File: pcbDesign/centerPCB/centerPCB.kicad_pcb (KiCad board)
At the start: 2 copper layers, 157 x 58.8 mm, 11 parts, among them J1 Conn_01x07_Pin, J2 Conn_01x12_Pin

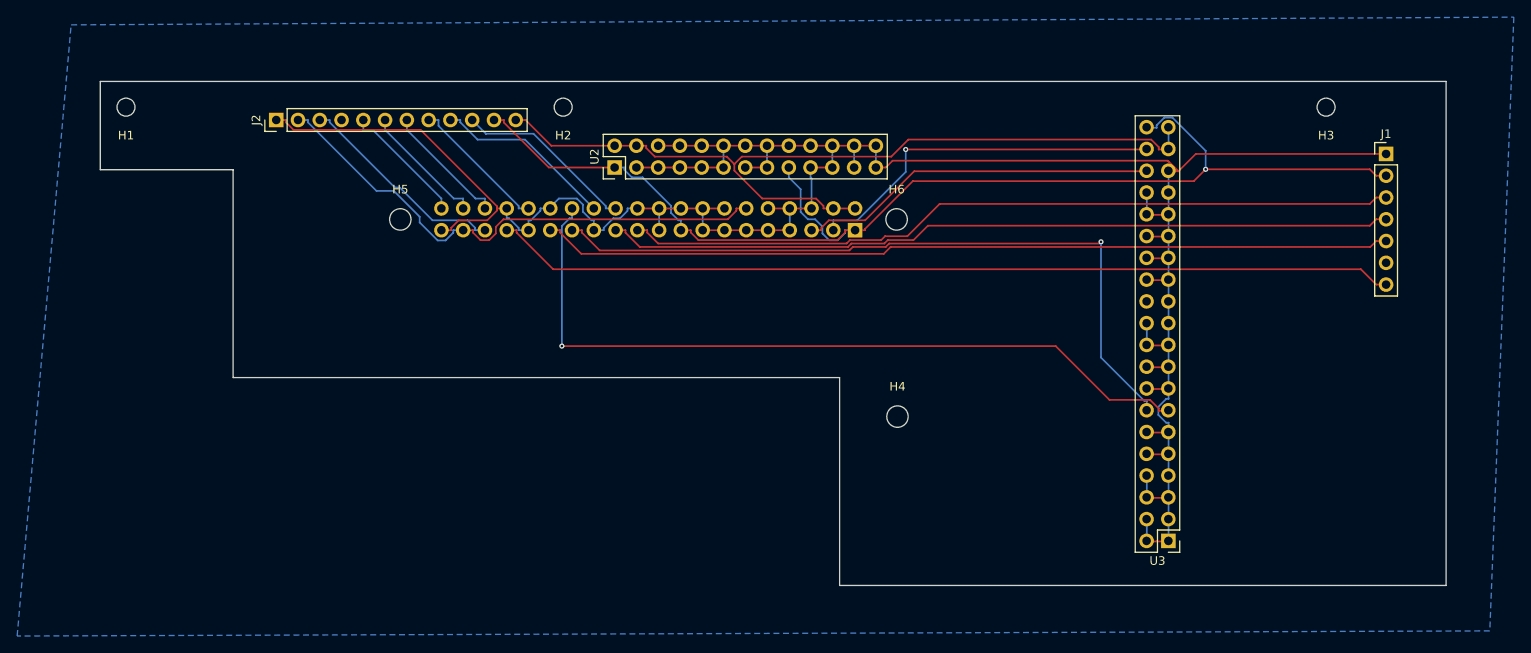
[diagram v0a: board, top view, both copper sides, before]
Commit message: rerouted
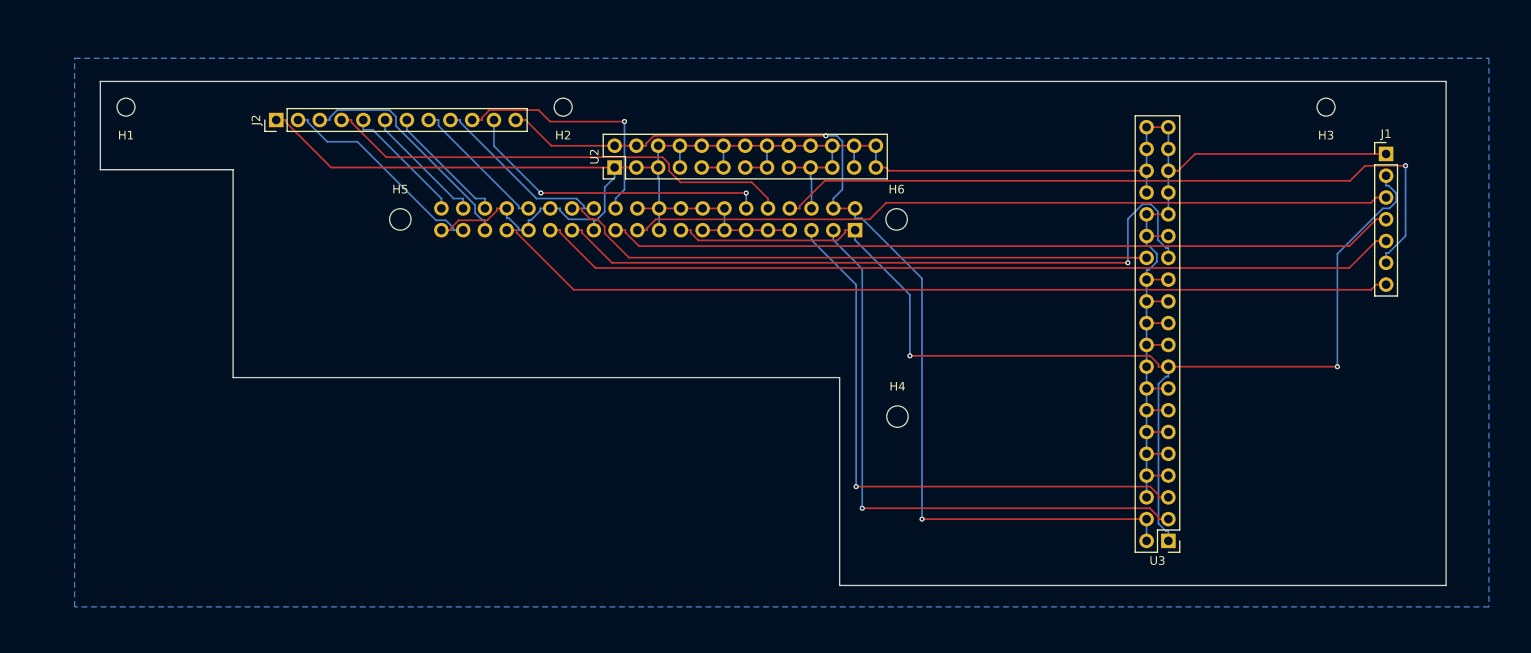
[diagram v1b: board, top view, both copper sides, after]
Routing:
- net /Brightness_B: track 0.00 -> 86.5 mm, vias 0 -> 1
- net /Volume_A: track 0.00 -> 55.3 mm
- net /Volume_B: track 62.1 -> 24.9 mm
- net /Clk: track 0.00 -> 36.5 mm, vias 0 -> 2
- net /MCU SDA: track 45.2 -> 70.2 mm
- net /MCU SCL: track 44.7 -> 69.2 mm, vias 0 -> 1
- net /5v: track 97.1 -> 119.7 mm, vias 0 -> 2
- net /EEPROM SDL: track 90.8 -> 70.0 mm, vias 1 -> 0
- net GND: track 289.0 -> 308.1 mm
- net /3v3: track 146.5 -> 137.4 mm, vias 1 -> 2
- net /Power_LED: track 21.2 -> 29.5 mm, vias 0 -> 1
- net /EEPROM SDA: track 87.9 -> 82.3 mm
- net /LR_Clk: track 24.9 -> 27.6 mm
- net /1: track 99.4 -> 100.8 mm
- net /Start: track 90.4 -> 89.1 mm
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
